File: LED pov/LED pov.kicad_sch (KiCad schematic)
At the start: 32 parts, among them J1 AVR, J2 BATTERY, SW1 SWITCH, U1 ATmega328P-AU, Y1 16 MHZ

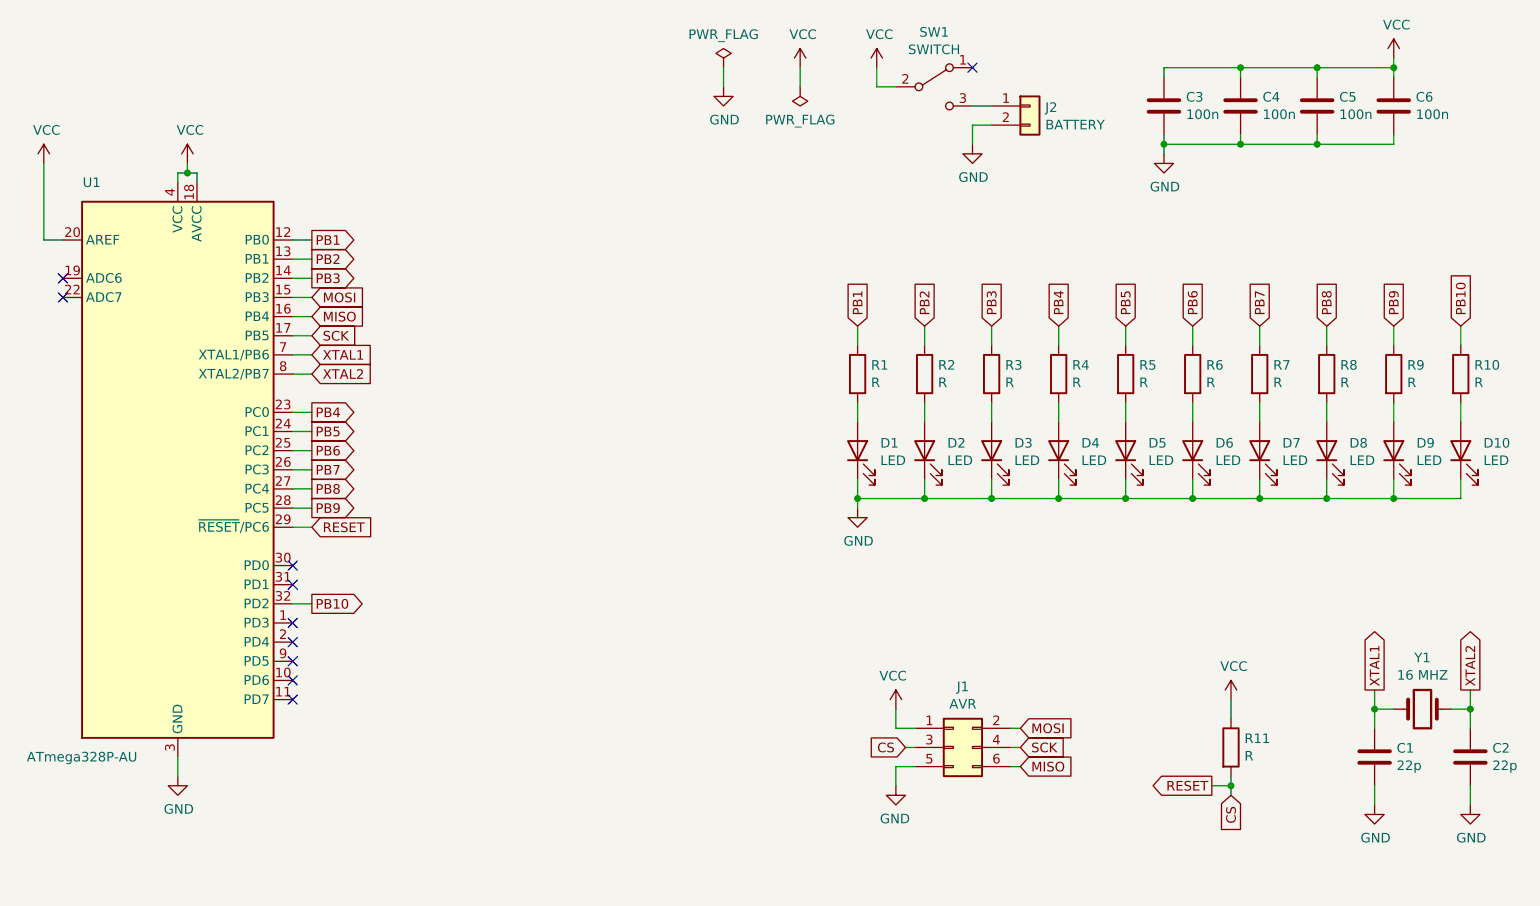
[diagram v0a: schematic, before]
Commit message: update files
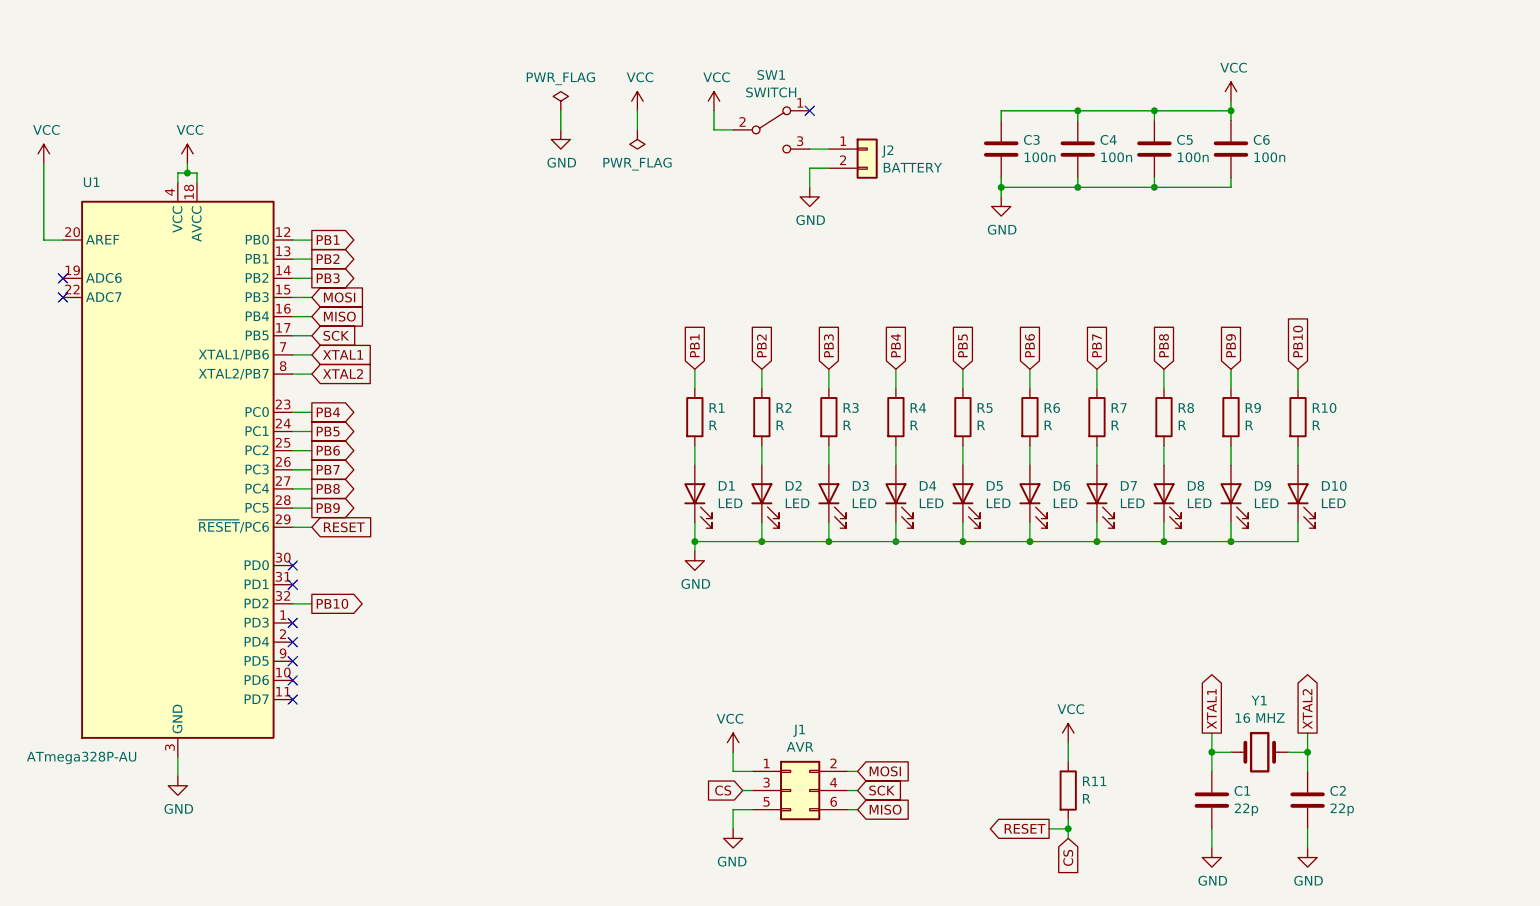
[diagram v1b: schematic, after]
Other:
- company: (none) -> Cristóbal Cuevas Lagos
- title: (none) -> LED pov
- moved on the sheet: C1, C2, C3, C4, C5, C6, D1, D10, D2, D3, D4, D5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
